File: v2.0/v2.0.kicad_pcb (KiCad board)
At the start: 2 copper layers, 145.5 x 88.5 mm, 50 parts, among them J1 MJ-4PP-9, SW1 SW_PUSH, SW10 SW_PUSH, SW11 SW_PUSH, SW12 SW_PUSH, SW13 SW_PUSH, SW14 SW_PUSH, SW15 SW_PUSH, SW16 SW_PUSH, SW17 SW_PUSH, SW18 SW_PUSH, SW19 SW_PUSH, SW2 SW_PUSH, SW20 SW_PUSH, SW21 SW_PUSH, SW22 SW_PUSH, SW3 SW_PUSH, SW4 SW_PUSH, SW5 SW_PUSH, SW6 SW_PUSH, SW7 SW_PUSH, SW8 SW_PUSH, SW9 SW_PUSH, U1 ProMicro, U2 switch

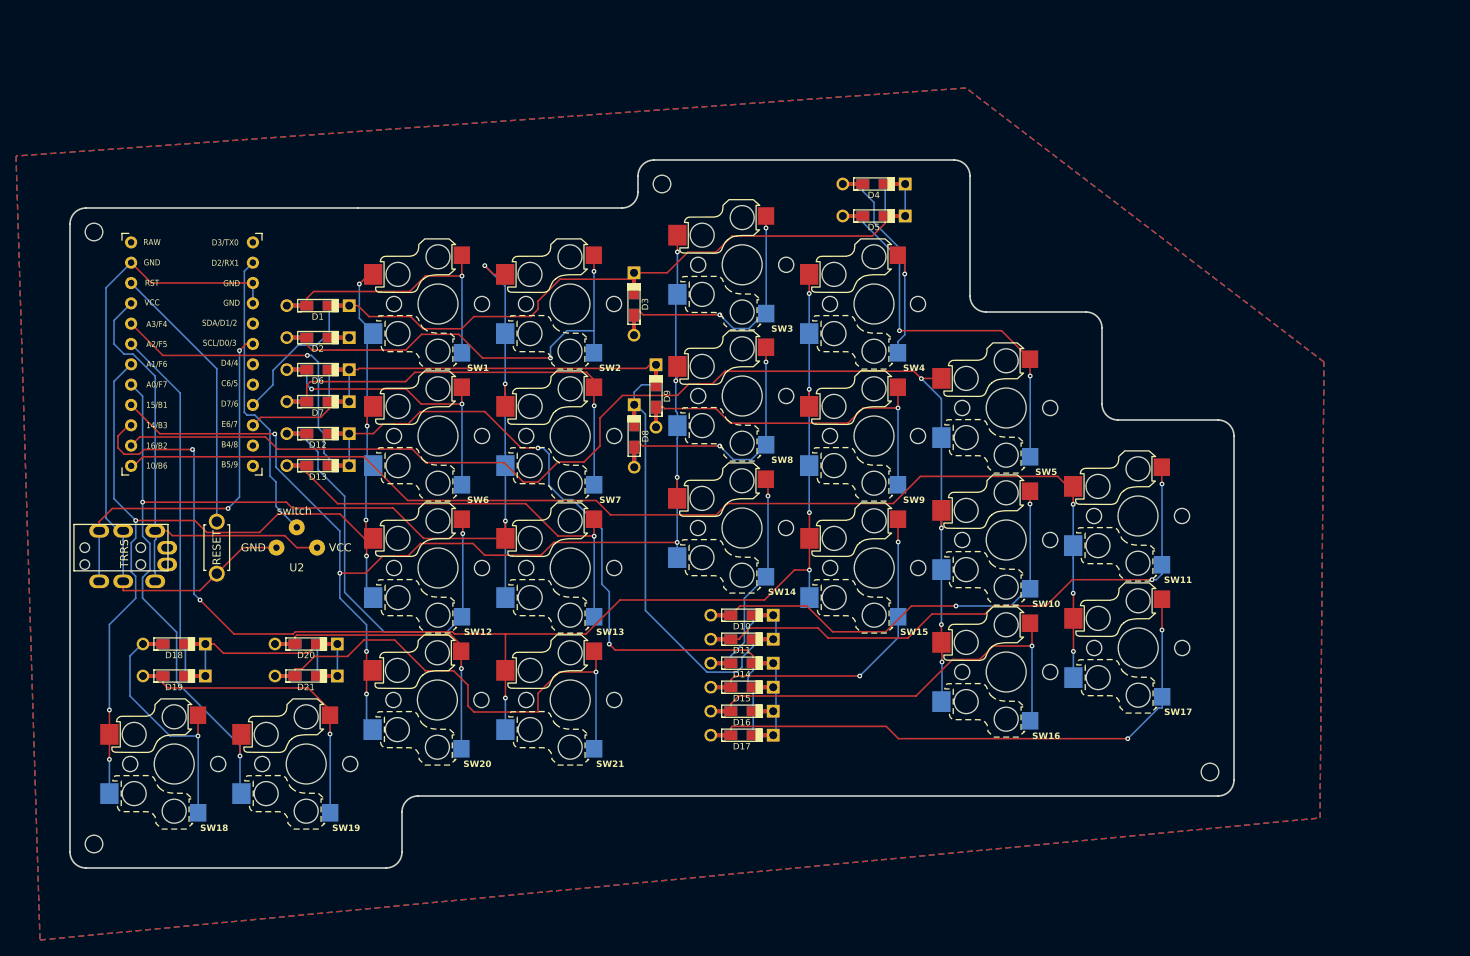
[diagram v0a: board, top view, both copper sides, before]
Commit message: updated
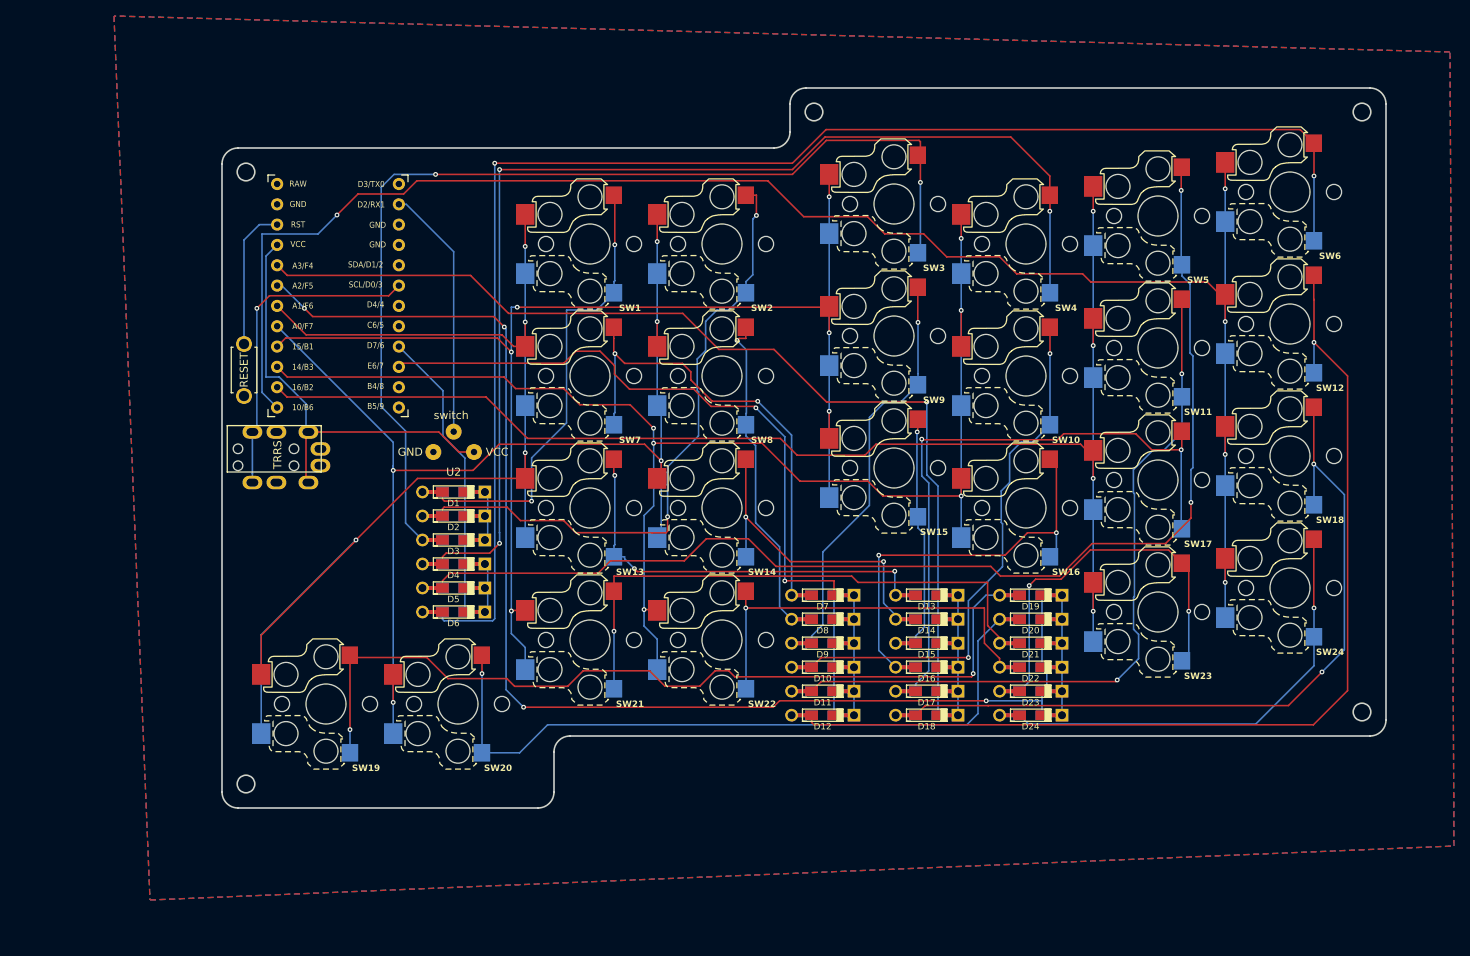
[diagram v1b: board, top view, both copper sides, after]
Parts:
- removed REF1, REF2, REF3, REF4: MountingHole_2.2mm_M2, MountingHole:MountingHole_2.2mm_M2
- added D22: D, Keebio-Parts:Diode-dual, F.Cu at (233.6, 142.4)
- added D23: D, Keebio-Parts:Diode-dual, F.Cu at (233.6, 145.4)
- added D24: D, Keebio-Parts:Diode-dual, F.Cu at (233.6, 148.4)
- added SW23: SW_PUSH, otborad:choc1_0.8u_reversible, F.Cu at (249.5, 135.5)
- added SW24: SW_PUSH, otborad:choc1_0.8u_reversible, F.Cu at (266.0, 132.5)
- added SW25: SW_PUSH, kbd:ResetSW, F.Cu at (135.2, 105.2)
- SW22: footprint kbd:ResetSW -> otborad:choc1_0.8u_reversible
- moved SW18 144.7 mm to (266.0, 116.0)
- moved SW12 110.8 mm to (266.0, 99.5)
- moved SW6 110.8 mm to (266.0, 83.0)
- moved D19 107.6 mm to (233.6, 133.4)
- moved D18 94.5 mm to (220.6, 148.4)
- moved D21 90.7 mm to (233.6, 139.4)
- moved D20 90.6 mm to (233.6, 136.4)
- moved D13 77.8 mm to (220.6, 133.4)
- moved D12 72.3 mm to (207.6, 148.4)
- moved D4 70.8 mm to (161.5, 129.5)
- moved D5 70.2 mm to (161.5, 132.5)
- moved D7 67.6 mm to (207.6, 133.4)
- moved SW22 64.2 mm to (195.0, 139.0), turned to 0 degrees
- moved D9 37.3 mm to (207.6, 139.4), turned to 0 degrees
- moved D3 37.1 mm to (161.5, 126.5), turned to 0 degrees
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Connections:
- D12 pad 1: row3 -> row2
- D18 pad 1: row4 -> row3
- D6 pad 1: row2 -> row1
- SW10 pad 1: col5 -> col4
- SW11 pad 1: col6 -> col5
- SW12 pad 1: col1 -> col6
- SW13 pad 1: col2 -> col1
- SW14 pad 1: col3 -> col2
- SW15 pad 1: col4 -> col3
- SW16 pad 1: col5 -> col4
- SW17 pad 1: col6 -> col5
- SW18 pad 1: col1 -> col6
- SW19 pad 1: col2 -> col1
- SW20 pad 1: col3 -> col2
- SW21 pad 1: col4 -> col3
- SW22 pad 1: reset -> col4
- SW22 pad 2: GND -> Net-(D22-A)
- SW6 pad 1: col1 -> col6
- SW7 pad 1: col2 -> col1
- SW8 pad 1: col3 -> col2
- SW9 pad 1: col4 -> col3
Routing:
- net Net-(D6-A): track 39.5 -> 186.6 mm
- net Net-(D4-A): track 31.2 -> 148.0 mm, vias 1 -> 3
- net row4: track 88.8 -> 203.7 mm, vias 0 -> 4
- net Net-(D5-A): track 51.2 -> 151.2 mm
- net Net-(D3-A): track 36.8 -> 135.1 mm
- net GND: track 83.9 -> 0.00 mm
- net Net-(D12-A): track 56.6 -> 132.3 mm
- net col6: track 147.9 -> 218.6 mm, vias 3 -> 5
- net Net-(D19-A): track 42.0 -> 111.3 mm, vias 1 -> 2
- net Net-(D18-A): track 37.7 -> 99.0 mm, vias 1 -> 2
- net Net-(D24-A): track 0.00 -> 61.1 mm, vias 0 -> 1
- net Net-(D22-A): track 0.00 -> 55.2 mm, vias 0 -> 1
- net Net-(D20-A): track 40.3 -> 94.2 mm
- net Net-(D23-A): track 0.00 -> 53.3 mm, vias 0 -> 2
- net row1: track 125.6 -> 75.2 mm
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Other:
- board size 145.5 x 88.5 mm -> 145.5 x 90 mm
